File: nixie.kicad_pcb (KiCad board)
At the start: 4 copper layers, 182.5 x 65.2 mm, 55 parts, among them IC1 SN74141, IC2 SN74141, IC3 SN74141, IC4 SN74141, IC5 MCP23017-E_SO, IC6 DS3231M+TRL, IC7 SN74141, IC8 SN74141, IC9 L7805CD2T-TR, J2 M20-9990646, J3 OSTVN02A150, J4 OSTVN02A150

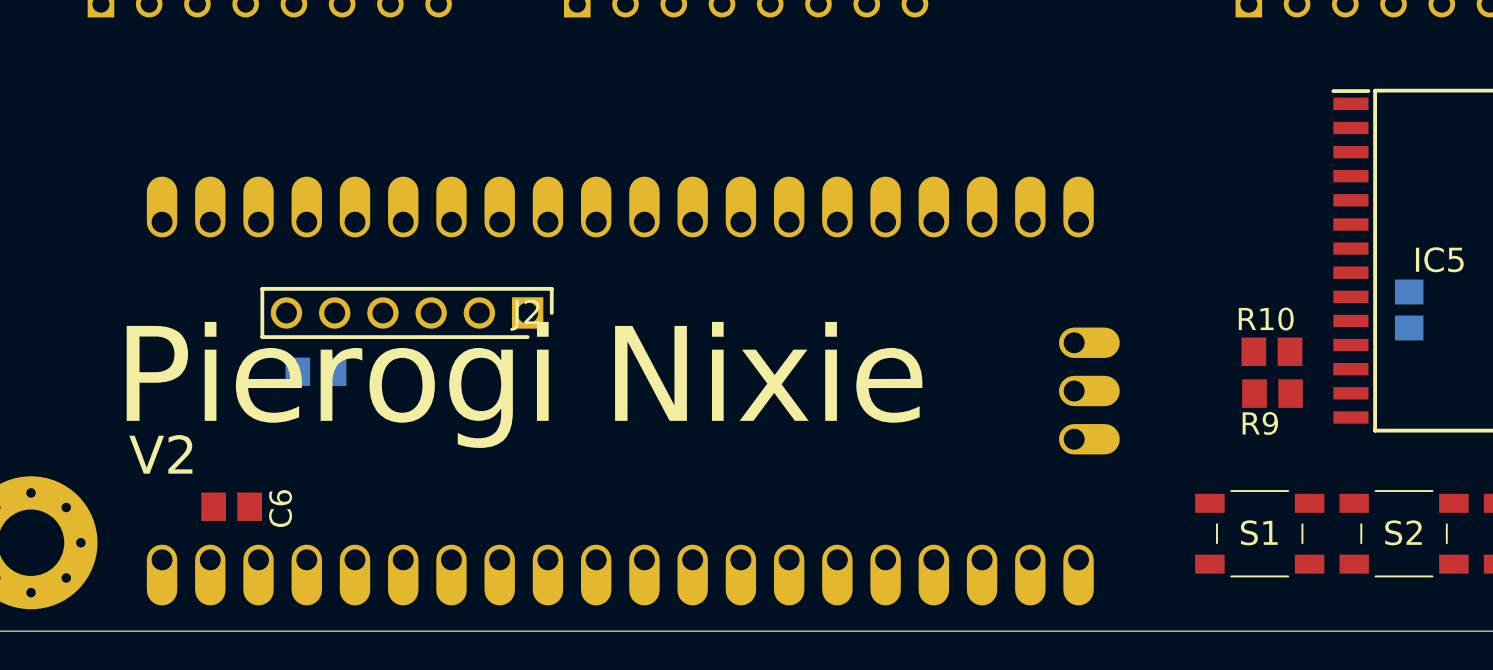
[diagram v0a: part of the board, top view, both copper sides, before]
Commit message: Changes to schematic
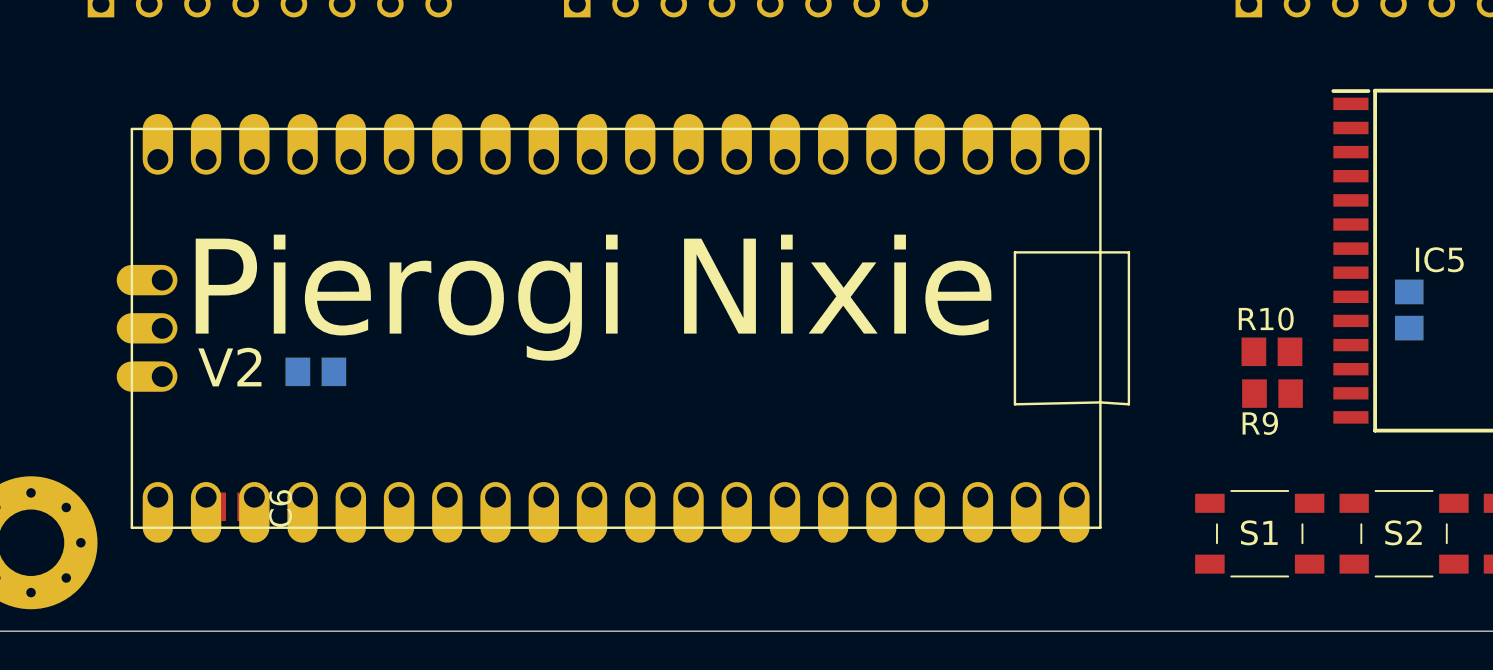
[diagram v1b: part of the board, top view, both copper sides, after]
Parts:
- removed J2: M20-9990646, footprints:HDRV6W64P0X254_1X6_1524X254X864P
- U$1: moved to F.Cu
- moved U$1 3.31 mm to (100.8, 127.1)
